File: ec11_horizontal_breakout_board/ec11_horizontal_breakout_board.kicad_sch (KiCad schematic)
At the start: 9 parts, among them J1 Conn_01x01_Socket, J2 Conn_01x01_Socket, J3 Conn_01x01_Socket, J4 Conn_01x01_Socket, J50 JST-SH-4, SW3 RotaryEncoder_Switch

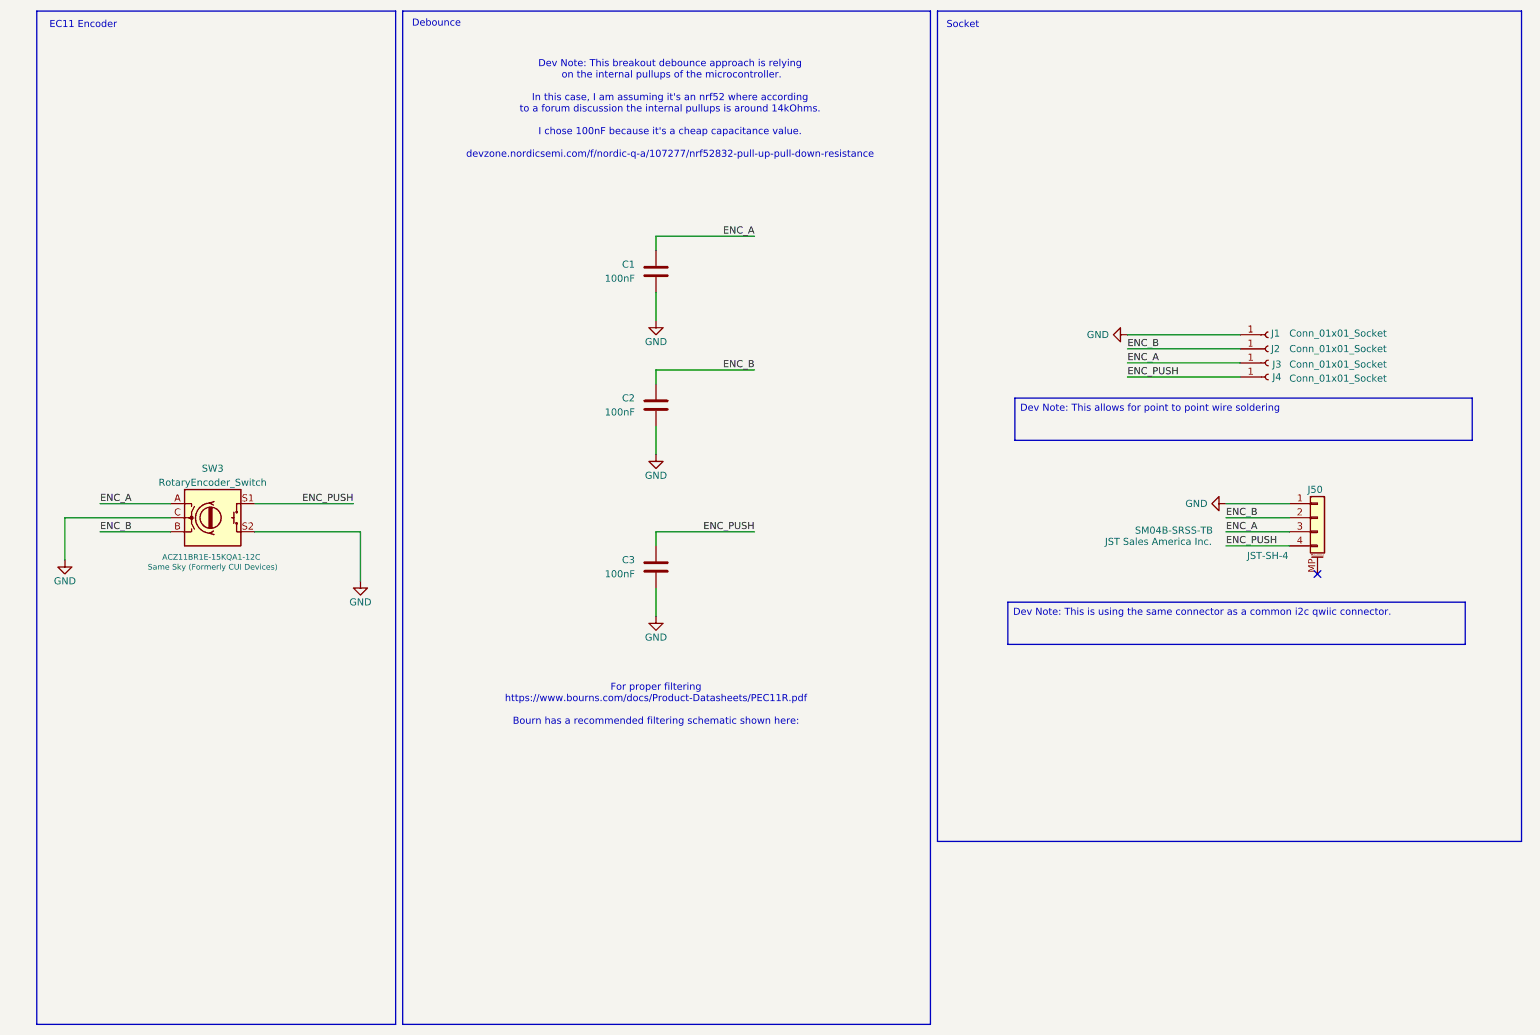
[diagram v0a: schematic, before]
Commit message: Ec11 breakout encoder Rev3
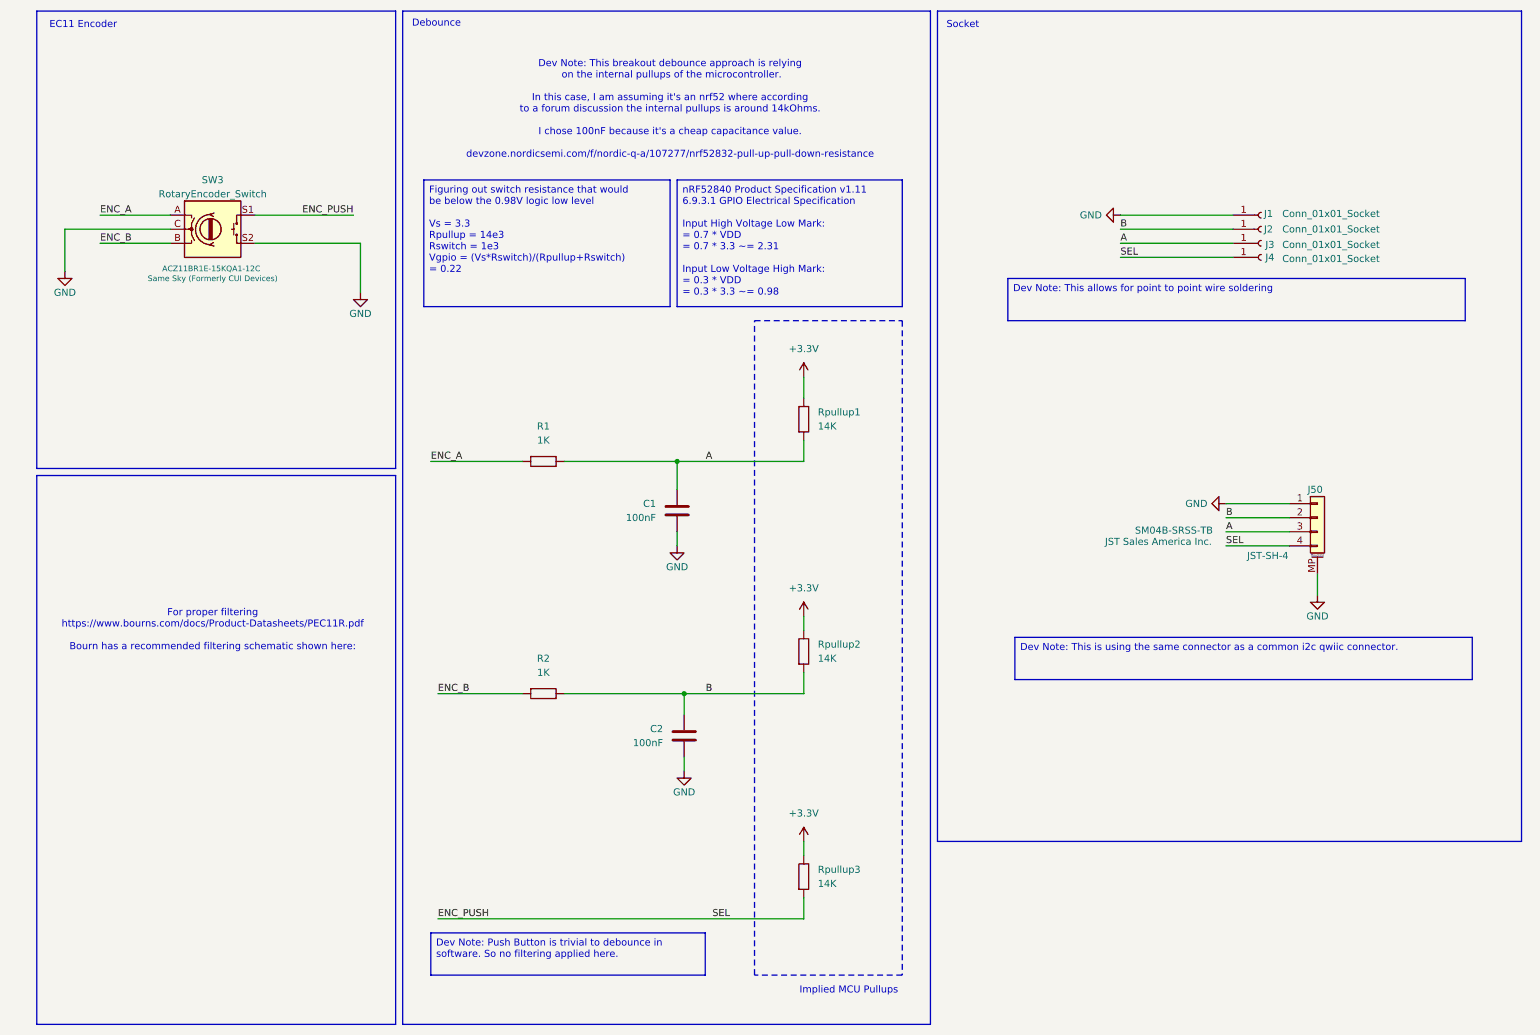
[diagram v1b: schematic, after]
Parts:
- removed C3: 100nF, Capacitor_SMD:C_0805_2012Metric_Pad1.18x1.45mm_HandSolder, symbol Device:C
- added R1, R2: 1K, EC11:R_0805_2012Metric_Pad1.20x1.40mm_HandSolder_And_Jumper, symbol PCM_SL_Resistors:Resistor
- added Rpullup1, Rpullup2, Rpullup3: 14K, Resistor_SMD:R_0805_2012Metric_Pad1.20x1.40mm_HandSolder, symbol PCM_SL_Resistors:Resistor
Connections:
- net ENC_A: now also R1.1; no longer C1.1, J3.1 (Pin_1), J50.3 (Pin_3)
- net ENC_B: now also R2.1; no longer C2.1, J2.1 (Pin_1), J50.2 (Pin_2)
- net ENC_PUSH: now also Rpullup3.1
- net GND: now also J50.MP (MountPin)
- new net +3.3V: Rpullup1.2, Rpullup2.2, Rpullup3.2
- new net A: C1.1, J3.1 (Pin_1), J50.3 (Pin_3), R1.2, Rpullup1.1
- new net B: C2.1, J2.1 (Pin_1), J50.2 (Pin_2), R2.2, Rpullup2.1
- no-connect marks 1 -> 0
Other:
- note added: "Implied MCU Pullups"
- moved on the sheet: C1, C2, J1, J2, J3, J4, SW3
